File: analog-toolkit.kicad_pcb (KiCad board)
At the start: 2 copper layers, 50 x 36 mm, 55 parts, among them J1 USB_C, J2 IO, J3 UART, J4 I2C, J5 VBUS, J6 3.3V, J7 OPAMP, J8 ADC, P1 TC2030, Q1 AO3400A, SW1 DFU, U1 AP2204R-3.3, U2 otter_USBLC6-4, U3 STM32G431xB

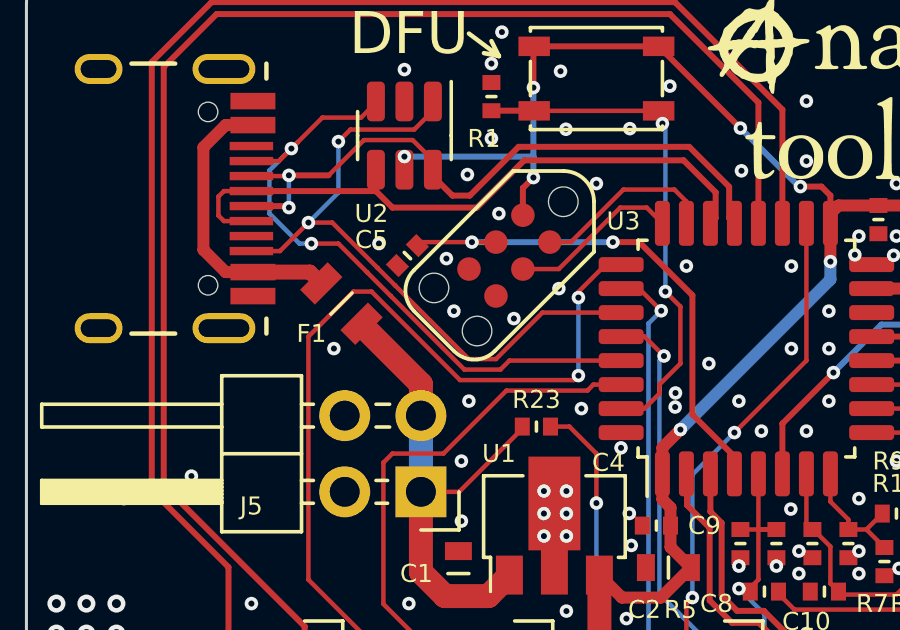
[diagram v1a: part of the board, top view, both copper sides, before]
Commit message: updated kicad files
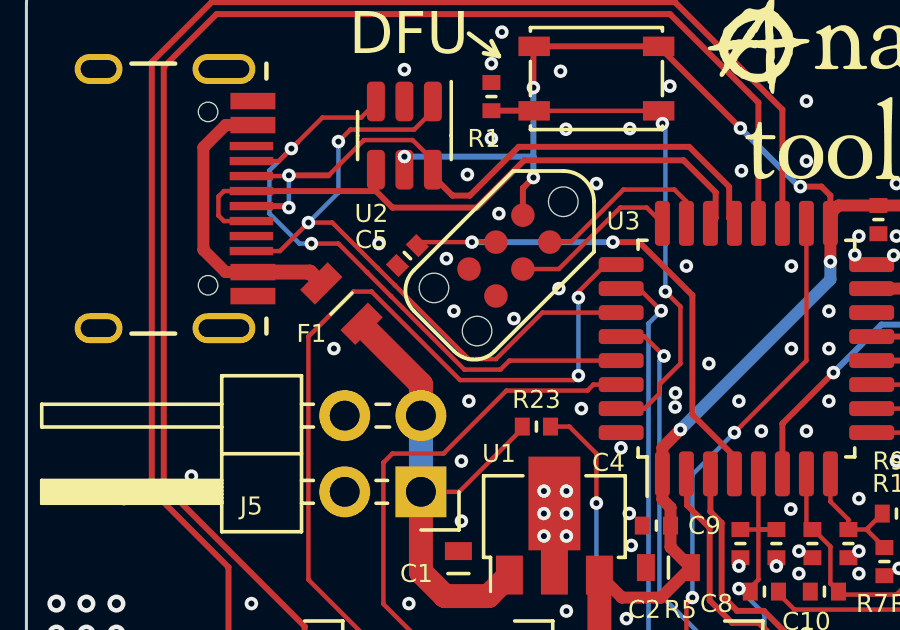
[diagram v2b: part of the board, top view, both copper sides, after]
